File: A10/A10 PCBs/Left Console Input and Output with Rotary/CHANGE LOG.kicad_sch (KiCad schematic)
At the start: 0 parts

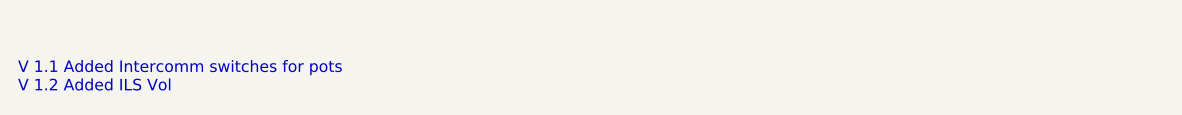
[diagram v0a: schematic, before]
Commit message: PCB
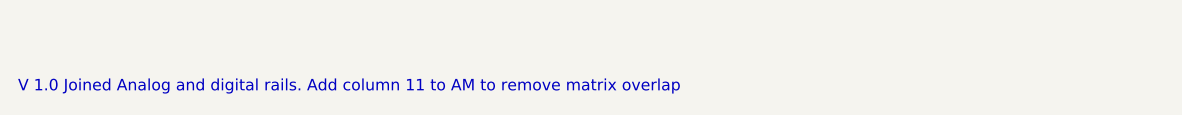
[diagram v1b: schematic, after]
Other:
- note added: "V 1.0 Joined Analog and digital rails. Add column 11 to AM to remove matrix overlap"
- note removed: "V 1.1 Added Intercomm switches for pots V 1.2 Added ILS Vol"
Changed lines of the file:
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@@
 		(date "2024-08-06")
 	)
-	(text "V 1.1 Added Intercomm switches for pots\nV 1.2 Added ILS Vol"
+	(text "V 1.0 Joined Analog and digital rails. Add column 11 to AM to remove matrix overlap"
 		(exclude_from_sim no)
 		(at 32.258 27.686 0)

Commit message: Left controller corrections
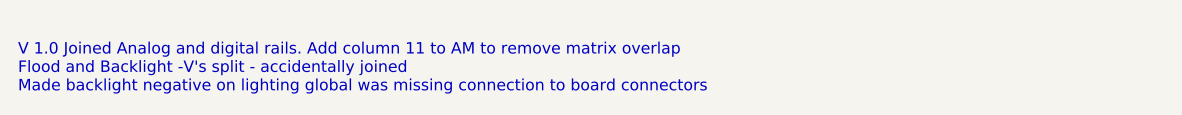
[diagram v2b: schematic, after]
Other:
- note added: "V 1.0 Joined Analog and digital rails. Add column 11 to AM to remove matrix overlap Flood and Backlight -V's split - accidentally joined Made backlight negative on lighting global was missing connection to board connectors"
- note removed: "V 1.0 Joined Analog and digital rails. Add column 11 to AM to remove matrix overlap"
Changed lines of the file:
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@@
 		(date "2024-08-06")
 	)
-	(text "V 1.0 Joined Analog and digital rails. Add column 11 to AM to remove matrix overlap"
+	(text "V 1.0 Joined Analog and digital rails. Add column 11 to AM to remove matrix overlap\nFlood and Backlight -V's split - accidentally joined\nMade backlight negative on lighting global was missing connection to board connectors"
 		(exclude_from_sim no)
 		(at 32.258 27.686 0)

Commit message: a10
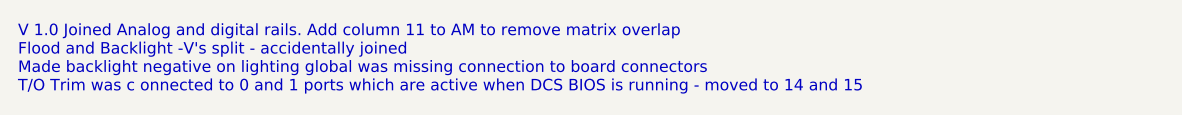
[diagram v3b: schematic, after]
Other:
- note added: "V 1.0 Joined Analog and digital rails. Add column 11 to AM to remove matrix overlap Flood and Backlight -V's split - accidentally joined Made backlight negative on lighting global was missing connection to board connectors T/O Trim was c onnected to 0 and 1 ports which are active when DCS BIOS is running - moved to 14 and 15"
- note removed: "V 1.0 Joined Analog and digital rails. Add column 11 to AM to remove matrix overlap Flood and Backlight -V's split - accidentally joined Made backlight negative on lighting global was missing connection to board connectors"
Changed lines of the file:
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@@
 		(date "2024-08-06")
 	)
-	(text "V 1.0 Joined Analog and digital rails. Add column 11 to AM to remove matrix overlap\nFlood and Backlight -V's split - accidentally joined\nMade backlight negative on lighting global was missing connection to board connectors"
+	(text "V 1.0 Joined Analog and digital rails. Add column 11 to AM to remove matrix overlap\nFlood and Backlight -V's split - accidentally joined\nMade backlight negative on lighting global was missing connection to board connectors\nT/O Trim was c onnected to 0 and 1 ports which are active when DCS BIOS is running - moved to 14 and 15"
 		(exclude_from_sim no)
 		(at 32.258 27.686 0)
